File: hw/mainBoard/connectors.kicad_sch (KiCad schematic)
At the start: 4 parts, among them J1 Conn_2Rows-39Pins, J2 UART_MODULE, J3 JTAG

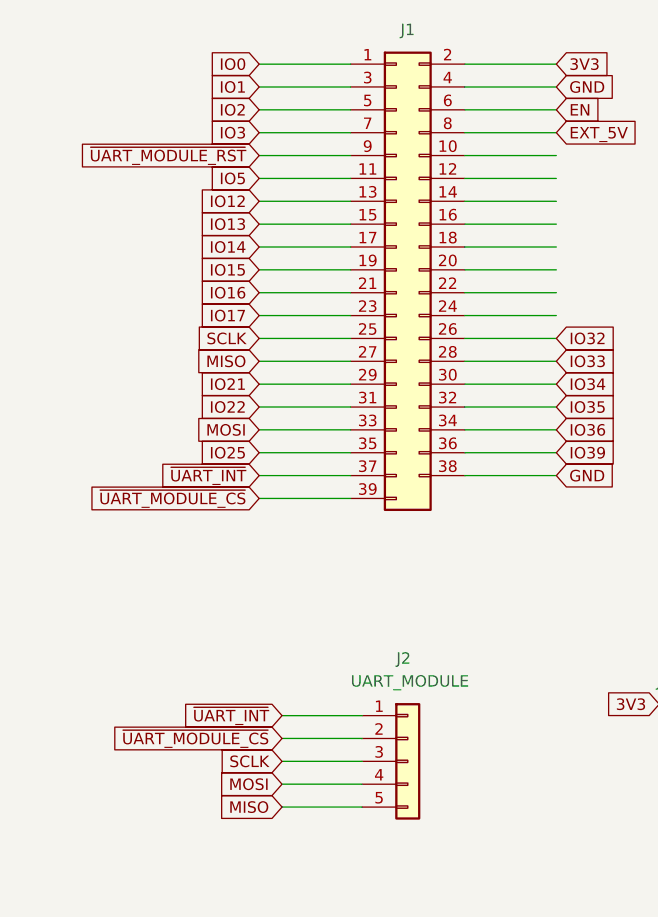
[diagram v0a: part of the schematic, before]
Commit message: hw
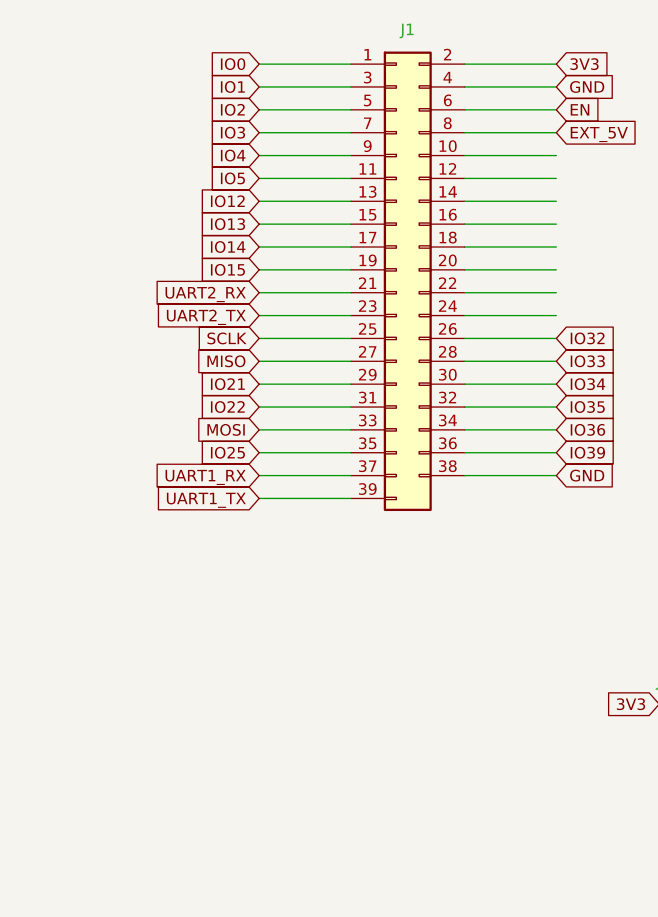
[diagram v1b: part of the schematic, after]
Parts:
- removed J2: UART_MODULE, symbol Connector_Generic:Conn_01x05
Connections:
- net IO16 renamed UART2_RX
- net IO17 renamed UART2_TX
- net ~{UART_INT} renamed UART1_RX
- net ~{UART_MODULE_CS} renamed UART1_TX
- net ~{UART_MODULE_RST} renamed IO4
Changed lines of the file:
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@@
-    (stroke (width 0) (type default))
-  )
-  (wire (pts (xy 104.14 120.65) (xy 113.03 120.65))
     (stroke (width 0) (type default))
   )
@@
     (stroke (width 0) (type default))
   )
-  (wire (pts (xy 104.14 130.81) (xy 113.03 130.81))
-    (stroke (width 0) (type default))
-  )
   (wire (pts (xy 173.99 119.38) (xy 181.61 119.38))
     (stroke (width 0) (type default))
@@
     (stroke (width 0) (type default))
   )
-  (wire (pts (xy 104.14 123.19) (xy 113.03 123.19))
-    (stroke (width 0) (type default))
-  )
   (wire (pts (xy 154.94 129.54) (xy 161.29 129.54))
     (stroke (width 0) (type default))
@@
     (stroke (width 0) (type default))
   )
-  (wire (pts (xy 104.14 128.27) (xy 113.03 128.27))
-    (stroke (width 0) (type default))
-  )
   (wire (pts (xy 101.6 53.34) (xy 111.76 53.34))
     (stroke (width 0) (type default))
@@
     (stroke (width 0) (type default))
   )
-  (wire (pts (xy 104.14 125.73) (xy 113.03 125.73))
-    (stroke (width 0) (type default))
-  )
   (wire (pts (xy 124.46 68.58) (xy 134.62 68.58))
     (stroke (width 0) (type default))
@@
     )
   )
-  (global_label "MOSI" (shape input) (at 104.14 128.27 180) (fields_autoplaced)
-    (effects (font (size 1.27 1.27)) (justify right))
-    (property "Intersheetrefs" "${INTERSHEET_REFS}" (at 96.8005 128.27 0)
-      (effects (font (size 1.27 1.27)) (justify right) hide)
-    )
-  )
   (global_label "MTDI" (shape input) (at 181.61 127 0) (fields_autoplaced)
     (effects (font (size 1.27 1.27)) (justify left))
@@
     )
   )
-  (global_label "MISO" (shape input) (at 104.14 130.81 180) (fields_autoplaced)
-    (effects (font (size 1.27 1.27)) (justify right))
-    (property "Intersheetrefs" "${INTERSHEET_REFS}" (at 96.8005 130.81 0)
-      (effects (font (size 1.27 1.27)) (justify right) hide)
-    )
-  )
   (global_label "IO12" (shape input) (at 101.6 63.5 180) (fields_autoplaced)
     (effects (font (size 1.27 1.27)) (justify right))
@@
     )
   )
-  (global_label "~{UART_INT}" (shape input) (at 104.14 120.65 180) (fields_autoplaced)
-    (effects (font (size 1.27 1.27)) (justify right))
-    (property "Intersheetrefs" "${INTERSHEET_REFS}" (at 96.8005 120.65 0)
-      (effects (font (size 1.27 1.27)) (justify right) hide)
-    )
-  )
   (global_label "GND" (shape input) (at 134.62 93.98 0) (fields_autoplaced)
     (effects (font (size 1.27 1.27)) (justify left))
@@
     )
   )
-  (global_label "IO17" (shape input) (at 101.6 76.2 180) (fields_autoplaced)
+  (global_label "UART2_TX" (shape input) (at 101.6 76.2 180) (fields_autoplaced)
     (effects (font (size 1.27 1.27)) (justify right))
     (property "Intersheetrefs" "${INTERSHEET_REFS}" (at 94.2605 76.2 0)
@@
     )
   )
-  (global_label "~{UART_MODULE_CS}" (shape input) (at 104.14 123.19 180) (fields_autoplaced)
-    (effects (font (size 1.27 1.27)) (justify right))
-    (property "Intersheetrefs" "${INTERSHEET_REFS}" (at 96.8005 123.19 0)
-      (effects (font (size 1.27 1.27)) (justify right) hide)
-    )
-  )
   (global_label "IO36" (shape input) (at 134.62 88.9 0) (fields_autoplaced)
     (effects (font (size 1.27 1.27)) (justify left))
@@
     )
   )
-  (global_label "~{UART_MODULE_CS}" (shape input) (at 101.6 96.52 180) (fields_autoplaced)
-    (effects (font (size 1.27 1.27)) (justify right))
-    (property "Intersheetrefs" "${INTERSHEET_REFS}" (at 94.2605 96.52 0)
-      (effects (font (size 1.27 1.27)) (justify right) hide)
-    )
-  )
-  (global_label "~{UART_INT}" (shape input) (at 101.6 93.98 180) (fields_autoplaced)
-    (effects (font (size 1.27 1.27)) (justify right))
-    (property "Intersheetrefs" "${INTERSHEET_REFS}" (at 94.2605 93.98 0)
+  (global_label "UART1_TX" (shape input) (at 101.6 96.52 180) (fields_autoplaced)
+    (effects (font (size 1.27 1.27)) (justify right))
+    (property "Intersheetrefs" "${INTERSHEET_REFS}" (at 89.6039 96.52 0)
+      (effects (font (size 1.27 1.27)) (justify right) hide)
+    )
+  )
+  (global_label "UART1_RX" (shape input) (at 101.6 93.98 180) (fields_autoplaced)
+    (effects (font (size 1.27 1.27)) (justify right))
+    (property "Intersheetrefs" "${INTERSHEET_REFS}" (at 89.3015 93.98 0)
       (effects (font (size 1.27 1.27)) (justify right) hide)
     )
@@
     )
   )
-  (global_label "~{UART_MODULE_RST}" (shape input) (at 101.6 58.42 180) (fields_autoplaced)
+  (global_label "IO4" (shape input) (at 101.6 58.42 180) (fields_autoplaced)
     (effects (font (size 1.27 1.27)) (justify right))
     (property "Intersheetrefs" "${INTERSHEET_REFS}" (at 95.47 58.42 0)
@@
     )
   )
-  (global_label "IO16" (shape input) (at 101.6 73.66 180) (fields_autoplaced)
+  (global_label "UART2_RX" (shape input) (at 101.6 73.66 180) (fields_autoplaced)
     (effects (font (size 1.27 1.27)) (justify right))
     (property "Intersheetrefs" "${INTERSHEET_REFS}" (at 94.2605 73.66 0)
@@
     (property "Intersheetrefs" "${INTERSHEET_REFS}" (at 141.9595 81.28 0)
       (effects (font (size 1.27 1.27)) (justify left) hide)
-    )
-  )
-  (global_label "SCLK" (shape input) (at 104.14 125.73 180) (fields_autoplaced)
-    (effects (font (size 1.27 1.27)) (justify right))
-    (property "Intersheetrefs" "${INTERSHEET_REFS}" (at 96.8005 125.73 0)
-      (effects (font (size 1.27 1.27)) (justify right) hide)
     )
   )
@@
         )
       )
-    )
-  )
-  (symbol (lib_id "Connector_Generic:Conn_01x05") (at 118.11 125.73 0) (unit 1)
-    (in_bom yes) (on_board yes) (dnp no)
-    (property "Reference" "J2" (at 116.84 114.3 0)
-      (effects (font (size 1.27 1.27)) (justify left))
-    )
-    (property "Value" "UART_MODULE" (at 111.76 116.84 0)
-      (effects (font (size 1.27 1.27)) (justify left))
-    )
-    (property "Footprint" "" (at 118.11 125.73 0)
-      (effects (font (size 1.27 1.27)) hide)
-    )
-    (property "Datasheet" "~" (at 118.11 125.73 0)
-      (effects (font (size 1.27 1.27)) hide)
-    )
-    (pin "1")
-    (pin "3")
-    (pin "4")
-    (pin "2")
-    (pin "5")
-    (instances
-      (project "mainBoard"
-        (path "/afbe4b5f-4e5c-4a12-a44b-208d158a3f7a/e09778c5-d723-4378-b78b-5054d4eb0fd5"
-          (reference "J2") (unit 1)
-        )
-      )

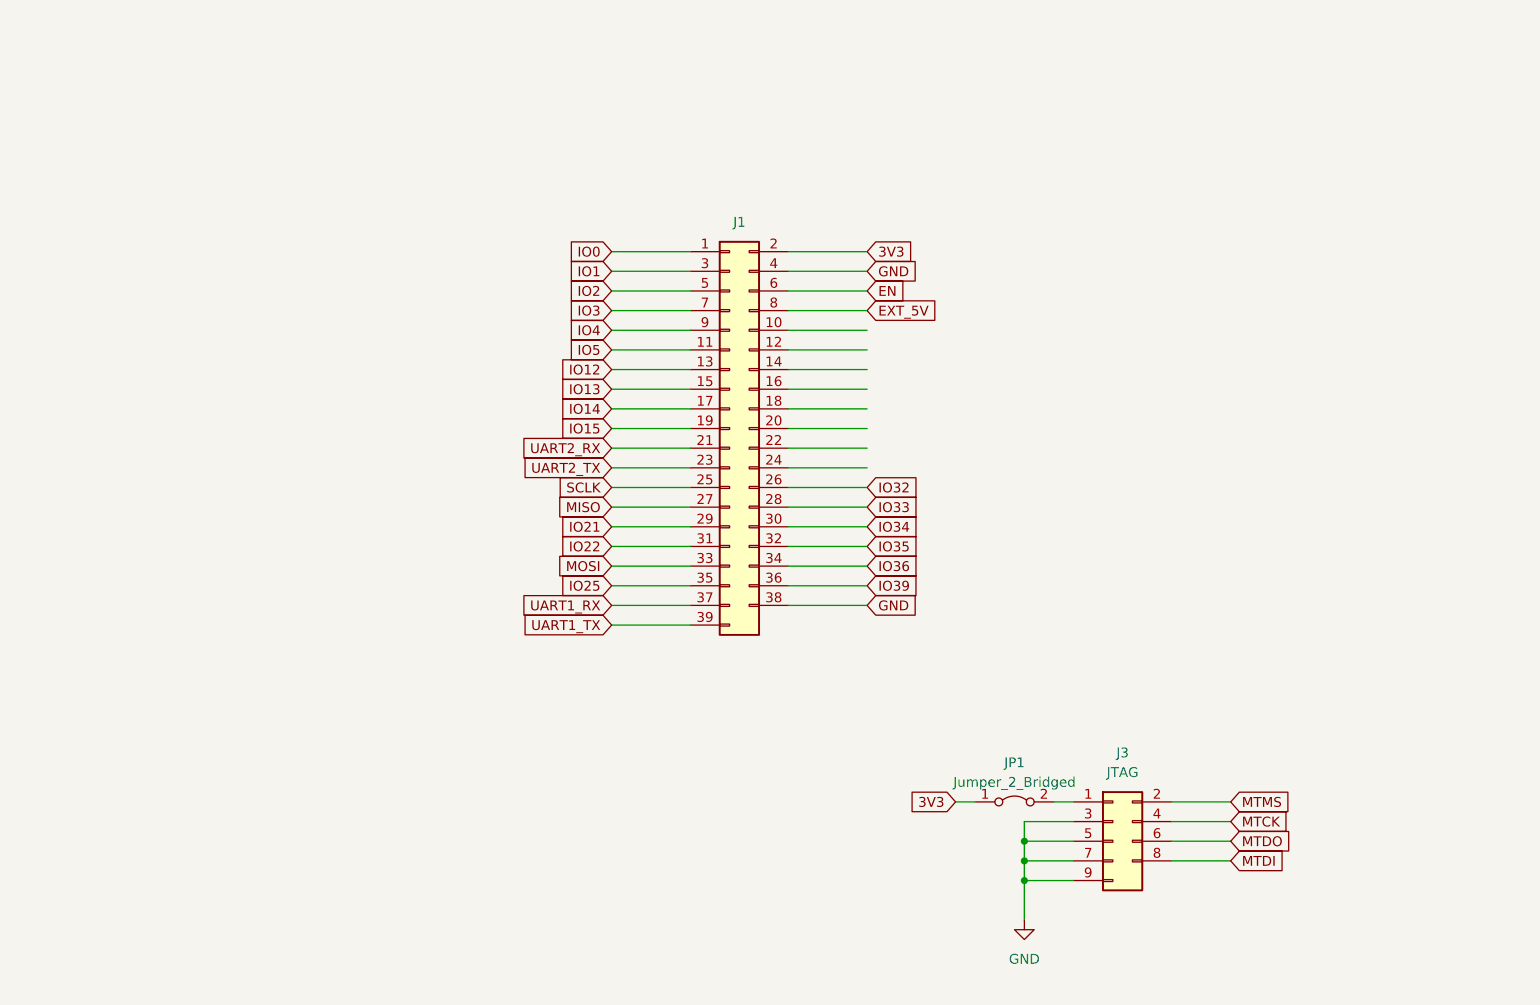
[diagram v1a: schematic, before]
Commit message: hw + blok schema
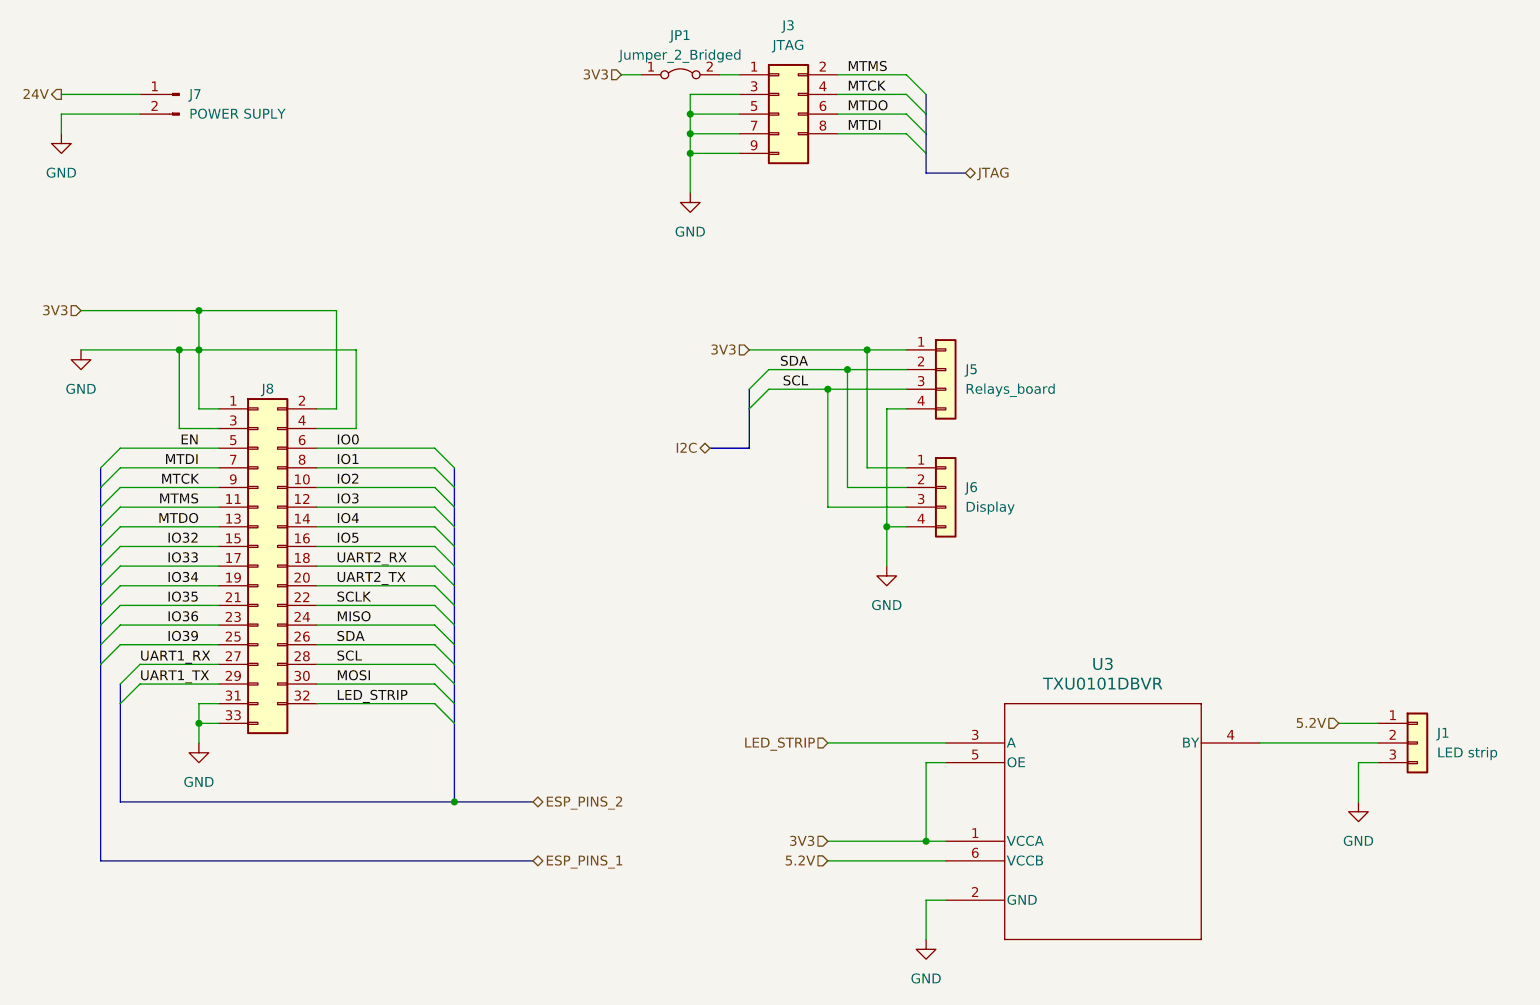
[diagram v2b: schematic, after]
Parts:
- removed J1: Conn_2Rows-39Pins, symbol Connector_Generic:Conn_2Rows-39Pins
- added J1: LED strip, symbol Connector_Generic:Conn_01x03
- added J5: Relays_board, Connector_JST:JST_XH_B4B-XH-AM_1x04_P2.50mm_Vertical, symbol Connector_Generic:Conn_01x04
- added J6: Display, Connector_JST:JST_XH_B4B-XH-AM_1x04_P2.50mm_Vertical, symbol Connector_Generic:Conn_01x04
- added J7: POWER SUPLY, symbol Connector:Conn_01x02_Pin
- added J8: Conn_2Rows-33Pins, symbol Connector_Generic:Conn_2Rows-33Pins
- added U3: TXU0101DBVR, SOT-23-6-DBV_TEX, symbol TXU0101:TXU0101DBVR
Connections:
- net 3V3 is gone; now on net GND: JP1.1 (A)
- net EN: now also J8.5 (Pin_5)
- net GND: now also J1.3 (Pin_3), J5.1 (Pin_1), J5.4 (Pin_4), J6.1 (Pin_1), J6.4 (Pin_4), J7.2 (Pin_2), J8.1 (Pin_1), J8.2 (Pin_2), J8.3 (Pin_3), J8.31 (Pin_31), J8.33 (Pin_33), J8.4 (Pin_4), U3.1 (VCCA), U3.2 (GND), U3.5 (OE)
- net IO0: now also J8.6 (Pin_6)
- net IO1: now also J8.8 (Pin_8)
- net IO2: now also J8.10 (Pin_10)
- net IO3: now also J8.12 (Pin_12)
- net IO32: now also J8.15 (Pin_15)
- net IO33: now also J8.17 (Pin_17)
- net IO34: now also J8.19 (Pin_19)
- net IO35: now also J8.21 (Pin_21)
- net IO36: now also J8.23 (Pin_23)
- net IO39: now also J8.25 (Pin_25)
- net IO4: now also J8.14 (Pin_14)
- net IO5: now also J8.16 (Pin_16)
- net MISO: now also J8.24 (Pin_24)
- net MOSI: now also J8.30 (Pin_30)
- net MTCK: now also J8.9 (Pin_9)
- net MTDI: now also J8.7 (Pin_7)
- net MTDO: now also J8.13 (Pin_13)
- net MTMS: now also J8.11 (Pin_11)
- net SCLK: now also J8.22 (Pin_22)
- net UART1_RX: now also J8.27 (Pin_27)
- net UART1_TX: now also J8.29 (Pin_29)
- net UART2_RX: now also J8.18 (Pin_18)
- net UART2_TX: now also J8.20 (Pin_20)
- new net: J1.2 (Pin_2), U3.4 (BY)
- new net 24V: J7.1 (Pin_1)
- new net 5.2V: J1.1 (Pin_1), U3.6 (VCCB)
- new net LED_STRIP: J8.32 (Pin_32), U3.3 (A)
- new net SCL: J5.3 (Pin_3), J6.3 (Pin_3), J8.28 (Pin_28)
- new net SDA: J5.2 (Pin_2), J6.2 (Pin_2), J8.26 (Pin_26)
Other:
- moved on the sheet: J3, JP1
